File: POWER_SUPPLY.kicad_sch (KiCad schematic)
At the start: 9 parts, among them J1 Jack-DC, U5 LM66100DCK, U6 LMR33640ADDA, U7 LMR33640ADDA

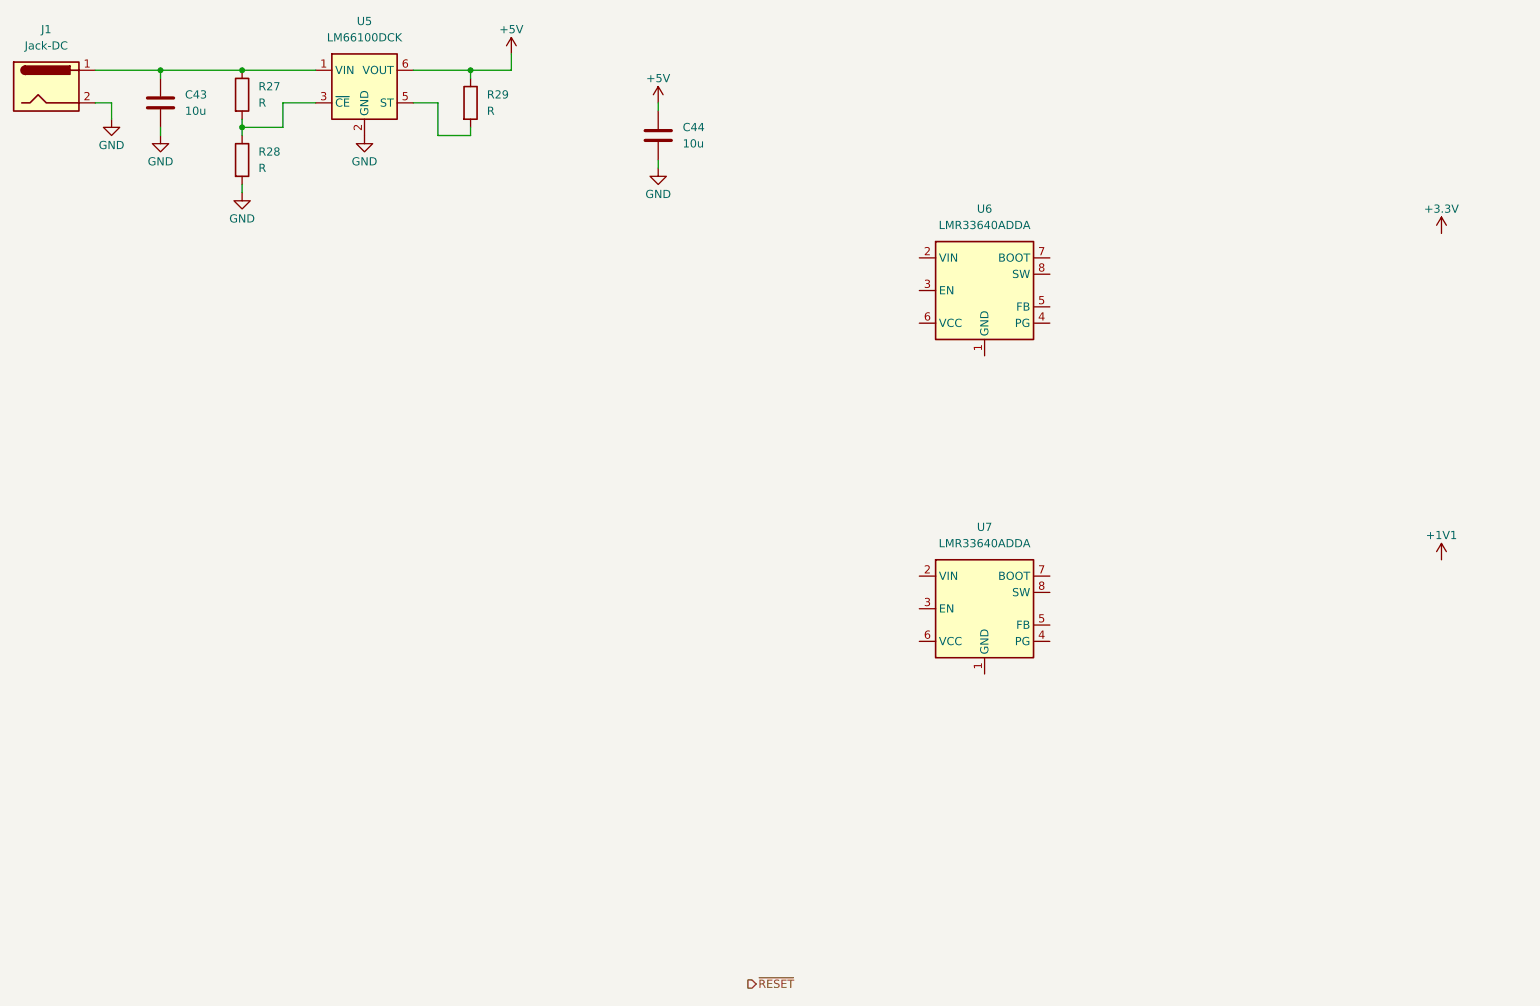
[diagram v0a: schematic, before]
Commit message: Weiter gemacht
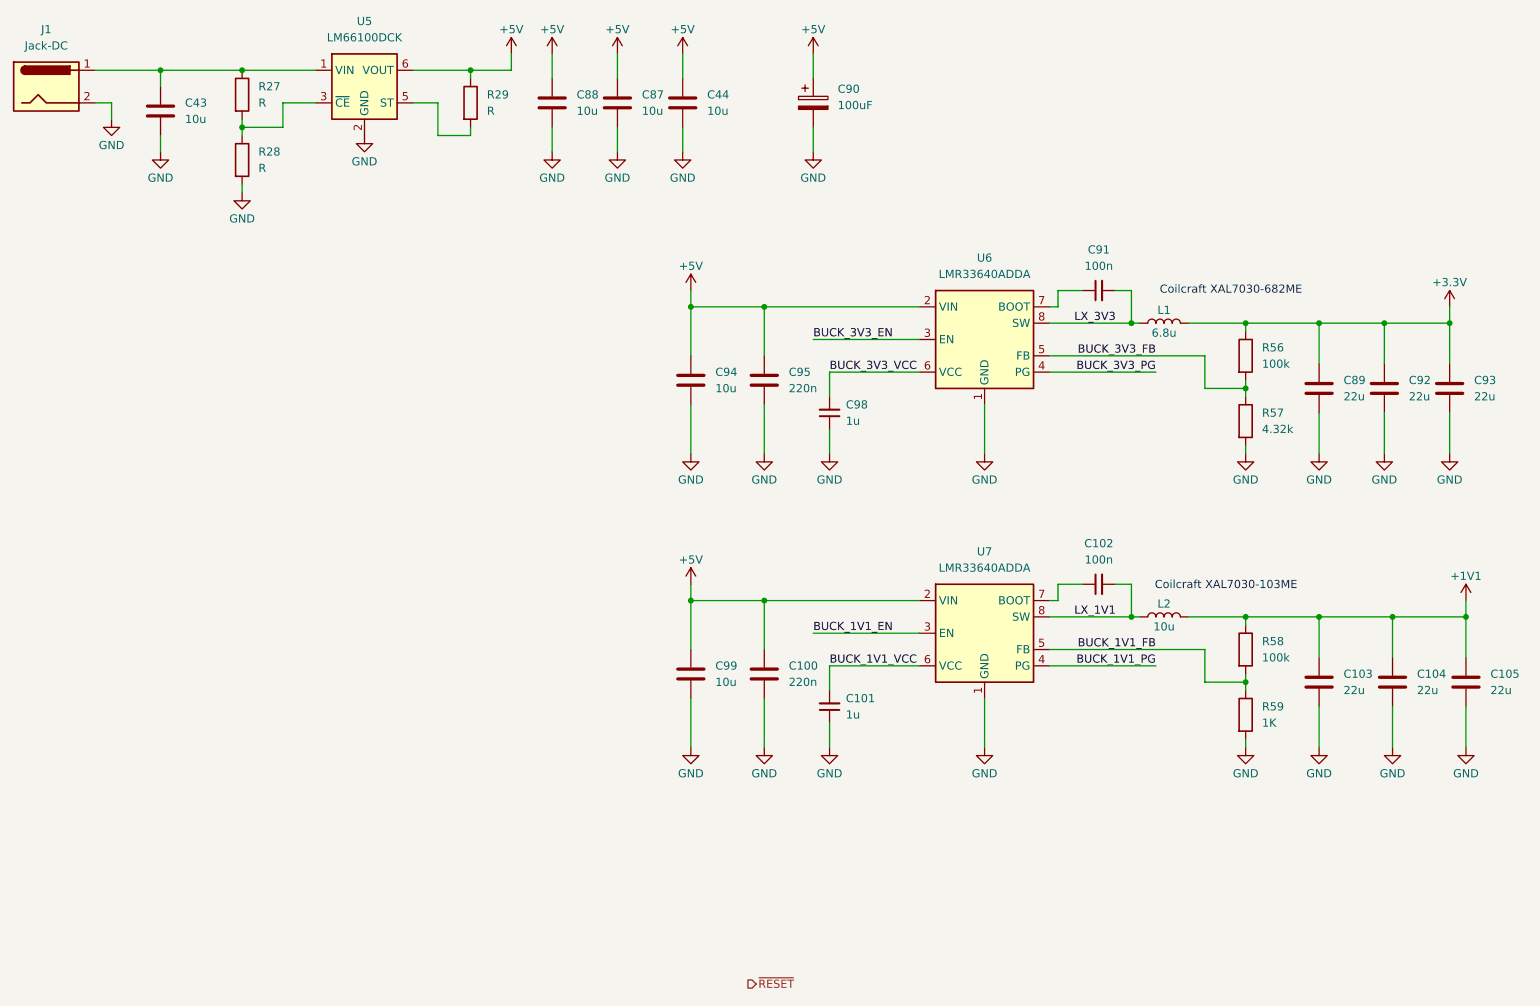
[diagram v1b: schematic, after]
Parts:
- added C100, C95: 220n, 00_Capacitor:Cap_0402, symbol Device:C
- added C101, C98: 1u, 00_Capacitor:Cap_0402, symbol Device:C_Small
- added C102, C91: 100n, 00_Capacitor:Cap_0402, symbol Device:C_Small
- added C103, C104, C105, C89, C92, C93: 22u, 00_Capacitor:Cap_0805, symbol Device:C
- added C87, C88, C94, C99: 10u, 00_Capacitor:Cap_0603, symbol Device:C
- added C90: 100uF, Capacitor_SMD:CP_Elec_6.3x5.9, symbol Device:C_Polarized
- added L1: 6.8u, Inductor_SMD:L_Coilcraft_XAL7030-272, symbol Device:L
- added L2: 10u, Inductor_SMD:L_Coilcraft_XAL7030-272, symbol Device:L
- added R56, R58: 100k, 00_Capacitor:Cap_0402, symbol Device:R
- added R57: 4.32k, 00_Capacitor:Cap_0402, symbol Device:R
- added R59: 1K, 00_Capacitor:Cap_0402, symbol Device:R
- J1: footprint (none) -> Connector_BarrelJack:BarrelJack_GCT_DCJ200-10-A_Horizontal
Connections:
- net +1V1: now also C103.1, C104.1, C105.1, L2.2, R58.1
- net +3.3V: now also C89.1, C92.1, C93.1, L1.2, R56.1
- net +5V: now also U6.2 (VIN), U7.2 (VIN), C100.1, C87.1, C88.1, C90.1, C94.1, C95.1, C99.1
- net GND: now also U6.1 (GND), U6.9 (GND), U7.1 (GND), U7.9 (GND), C100.2, C101.1, C103.2, C104.2, C105.2, C87.2, C88.2, C89.2, C90.2, C92.2, C93.2, C94.2, C95.2, C98.1, C99.2, R57.2, R59.2
- net BUCK_1V1_EN: now reaches U7.3 (EN)
- net BUCK_1V1_PG: now reaches U7.4 (PG)
- net BUCK_1V1_FB: now reaches U7.5 (FB)
- net BUCK_1V1_FB: now also R58.2, R59.1
- net BUCK_1V1_VCC: now reaches U7.6 (VCC)
- net BUCK_1V1_VCC: now also C101.2
- net at U7.7 (BOOT): now also C102.1
- net LX_1V1: now reaches U7.8 (SW)
- net LX_1V1: now also C102.2, L2.1
- net BUCK_3V3_EN: now reaches U6.3 (EN)
- net BUCK_3V3_PG: now reaches U6.4 (PG)
- net BUCK_3V3_FB: now reaches U6.5 (FB)
- net BUCK_3V3_FB: now also R56.2, R57.1
- net BUCK_3V3_VCC: now reaches U6.6 (VCC)
- net BUCK_3V3_VCC: now also C98.2
- net at U6.7 (BOOT): now also C91.1
- net LX_3V3: now reaches U6.8 (SW)
- net LX_3V3: now also C91.2, L1.1
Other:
- note added: "Coilcraft XAL7030-103ME"
- note added: "Coilcraft XAL7030-682ME"
- moved on the sheet: C43, C44, U6, U7
